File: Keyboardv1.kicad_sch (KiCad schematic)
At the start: 168 parts, among them SW1 SW_Push_45deg, SW10 SW_Push_45deg, SW11 SW_Push_45deg, SW12 SW_Push_45deg, SW13 SW_Push_45deg, SW14 SW_Push_45deg, SW15 SW_Push_45deg, SW16 SW_Push_45deg, SW17 SW_Push_45deg, SW18 SW_Push_45deg, SW19 SW_Push_45deg, SW2 SW_Push_45deg, SW20 SW_Push_45deg, SW21 SW_Push_45deg, SW22 SW_Push_45deg, SW23 SW_Push_45deg, SW24 SW_Push_45deg, SW25 SW_Push_45deg, SW26 SW_Push_45deg, SW27 SW_Push_45deg, SW28 SW_Push_45deg, SW29 SW_Push_45deg, SW3 SW_Push_45deg, SW30 SW_Push_45deg, SW31 SW_Push_45deg, SW32 SW_Push_45deg, SW33 SW_Push_45deg, SW34 SW_Push_45deg, SW35 SW_Push_45deg, SW36 SW_Push_45deg, SW37 SW_Push_45deg, SW38 SW_Push_45deg, SW39 SW_Push_45deg, SW4 SW_Push_45deg, SW40 SW_Push_45deg, SW41 SW_Push_45deg, SW42 SW_Push_45deg, SW43 SW_Push_45deg, SW44 SW_Push_45deg, SW45 SW_Push_45deg, SW46 SW_Push_45deg, SW47 SW_Push_45deg, SW48 SW_Push_45deg, SW49 SW_Push_45deg, SW5 SW_Push_45deg, SW50 SW_Push_45deg, SW51 SW_Push_45deg, SW52 SW_Push_45deg, SW53 SW_Push_45deg, SW54 SW_Push_45deg, SW55 SW_Push_45deg, SW56 SW_Push_45deg, SW57 SW_Push_45deg, SW58 SW_Push_45deg, SW59 SW_Push_45deg, SW6 SW_Push_45deg, SW60 SW_Push_45deg, SW61 SW_Push_45deg, SW62 SW_Push_45deg, SW63 SW_Push_45deg, SW64 SW_Push_45deg, SW65 SW_Push_45deg, SW66 SW_Push_45deg, SW67 SW_Push_45deg, SW68 SW_Push_45deg, SW69 SW_Push_45deg, SW7 SW_Push_45deg, SW70 SW_Push_45deg, SW71 SW_Push_45deg, SW72 SW_Push_45deg, SW73 SW_Push_45deg, SW74 SW_Push_45deg, SW75 SW_Push_45deg, SW76 SW_Push_45deg, SW77 SW_Push_45deg, SW78 SW_Push_45deg, SW79 SW_Push_45deg, SW8 SW_Push_45deg, SW80 SW_Push_45deg, SW81 SW_Push_45deg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

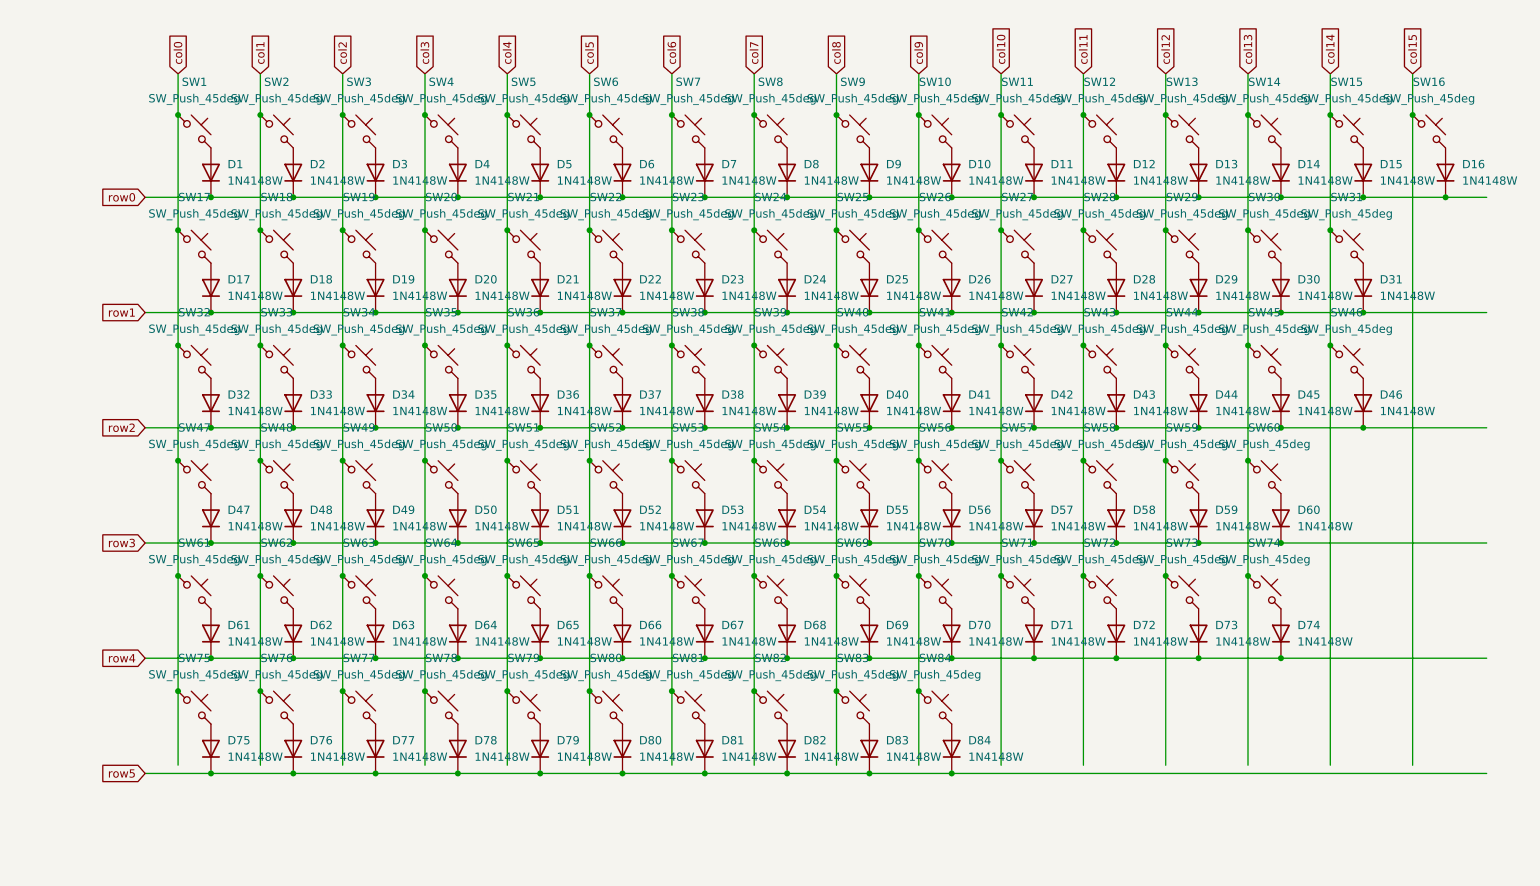
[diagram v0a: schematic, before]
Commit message: update
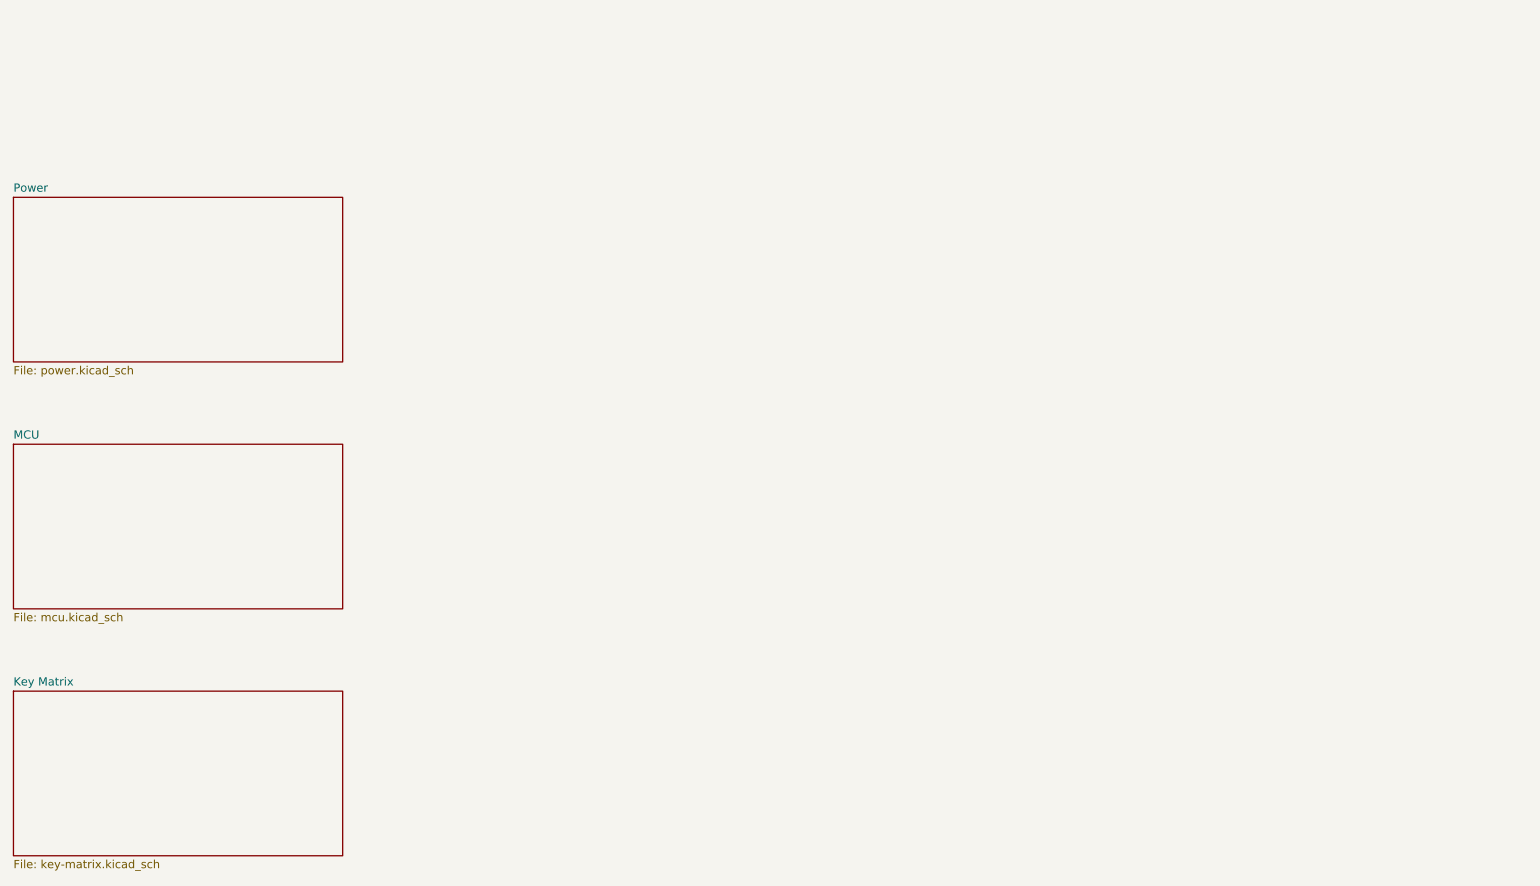
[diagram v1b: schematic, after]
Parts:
- removed D1, D10, D11, D12, D13, D14, D15, D16, D17, D18, D19, D2, D20, D21, D22, D23, D24, D25, D26, D27, D28, D29, D3, D30, D31, D32, D33, D34, D35, D36, D37, D38, D39, D4, D40, D41, D42, D43, D44, D45, D46, D47, D48, D49, D5, D50, D51, D52, D53, D54, D55, D56, D57, D58, D59, D6, D60, D61, D62, D63, D64, D65, D66, D67, D68, D69, D7, D70, D71, D72, D73, D74, D75, D76, D77, D78, D79, D8, D80, D81, D82, D83, D84, D9: 1N4148W, Diode_SMD:D_SOD-123, symbol Diode:1N4148W
- removed SW1, SW10, SW11, SW12, SW13, SW14, SW15, SW16, SW17, SW18, SW19, SW2, SW20, SW21, SW22, SW23, SW24, SW25, SW26, SW27, SW28, SW29, SW3, SW30, SW31, SW32, SW33, SW34, SW35, SW36, SW37, SW38, SW39, SW4, SW40, SW41, SW42, SW43, SW44, SW45, SW46, SW47, SW48, SW49, SW5, SW50, SW51, SW52, SW53, SW54, SW55, SW56, SW57, SW58, SW59, SW6, SW60, SW61, SW62, SW63, SW64, SW65, SW66, SW67, SW68, SW69, SW7, SW70, SW71, SW72, SW73, SW74, SW75, SW76, SW77, SW78, SW79, SW8, SW80, SW81, SW82, SW83, SW84, SW9: SW_Push_45deg, PCM_Switch_Keyboard_Cherry_MX:SW_Cherry_MX_PCB, symbol Switch:SW_Push_45deg
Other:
- added sheet Key Matrix (key-matrix.kicad_sch)
- added sheet MCU (mcu.kicad_sch)
- added sheet Power (power.kicad_sch)
